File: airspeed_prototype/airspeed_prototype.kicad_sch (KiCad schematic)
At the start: 2 parts, among them U1 BME280, U2 ADXL343

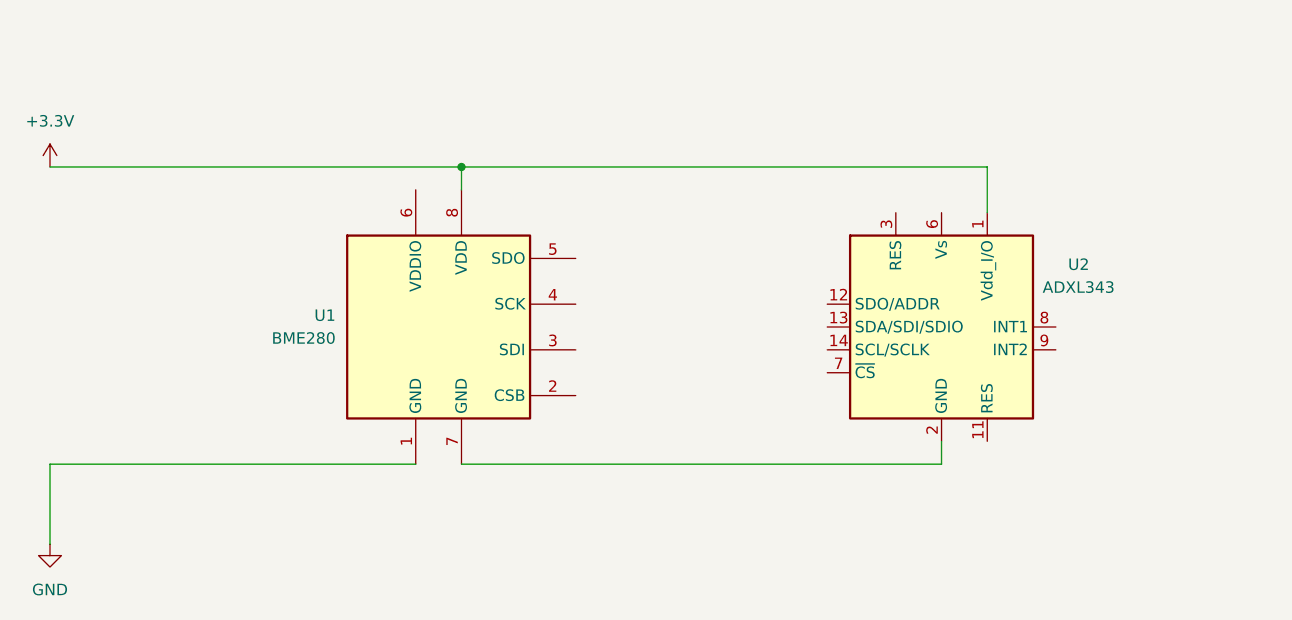
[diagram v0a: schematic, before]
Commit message: schematic
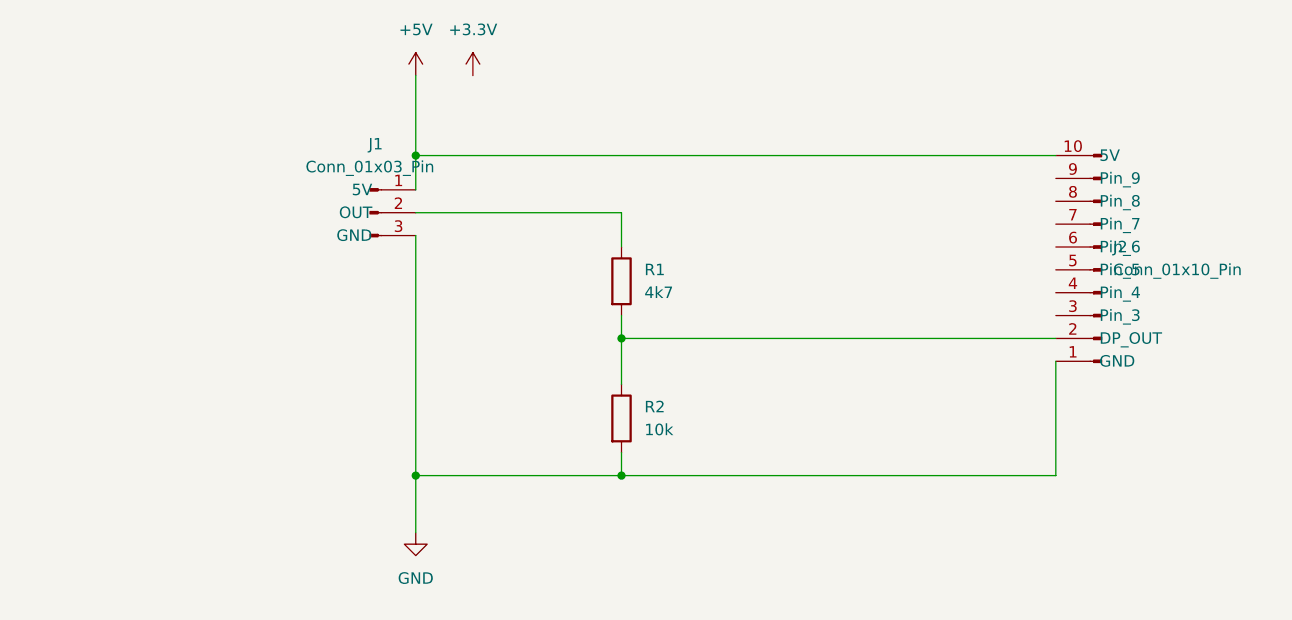
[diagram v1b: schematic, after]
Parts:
- removed U1: BME280, Package_LGA:Bosch_LGA-8_2.5x2.5mm_P0.65mm_ClockwisePinNumbering, symbol Sensor:BME280
- removed U2: ADXL343, Package_LGA:LGA-14_3x5mm_P0.8mm_LayoutBorder1x6y, symbol Sensor_Motion:ADXL343
- added J1: Conn_01x03_Pin, Connector_PinHeader_2.54mm:PinHeader_1x03_P2.54mm_Vertical, symbol Connector:Conn_01x03_Pin
- added J2: Conn_01x10_Pin, Connector_PinHeader_2.54mm:PinHeader_1x10_P2.54mm_Vertical, symbol Connector:Conn_01x10_Pin
- added R1: 4k7, Resistor_SMD:R_0805_2012Metric, symbol Device:R
- added R2: 10k, Resistor_SMD:R_0805_2012Metric, symbol Device:R
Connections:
- net GND: now also J1.3 (Pin_3), J2.1 (Pin_1), R2.2
- new net: J1.2 (Pin_2), R1.1
- new net: J2.2 (Pin_2), R1.2, R2.1
- new net +5V: J1.1 (Pin_1), J2.10 (Pin_10)

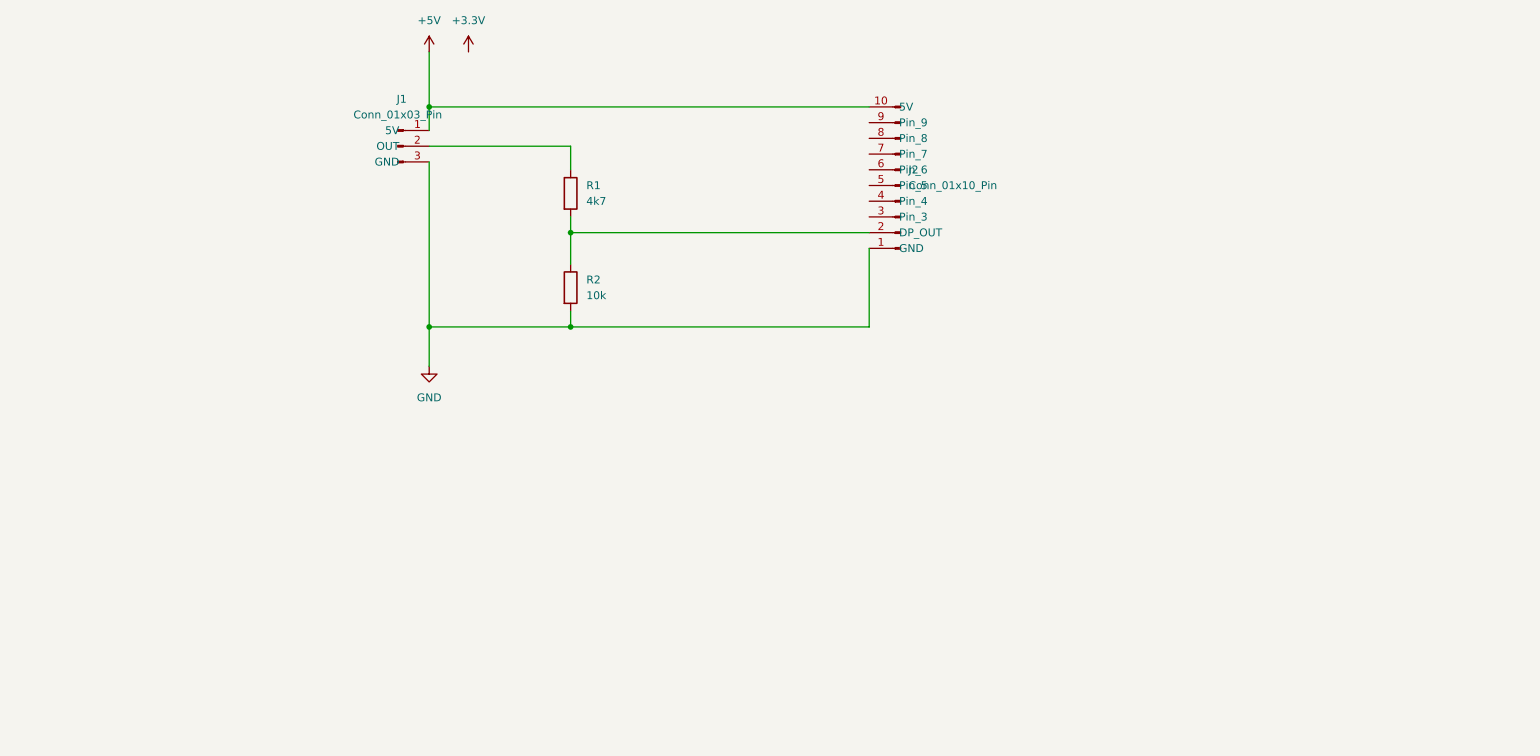
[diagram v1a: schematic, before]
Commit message: update the schematic and pcb
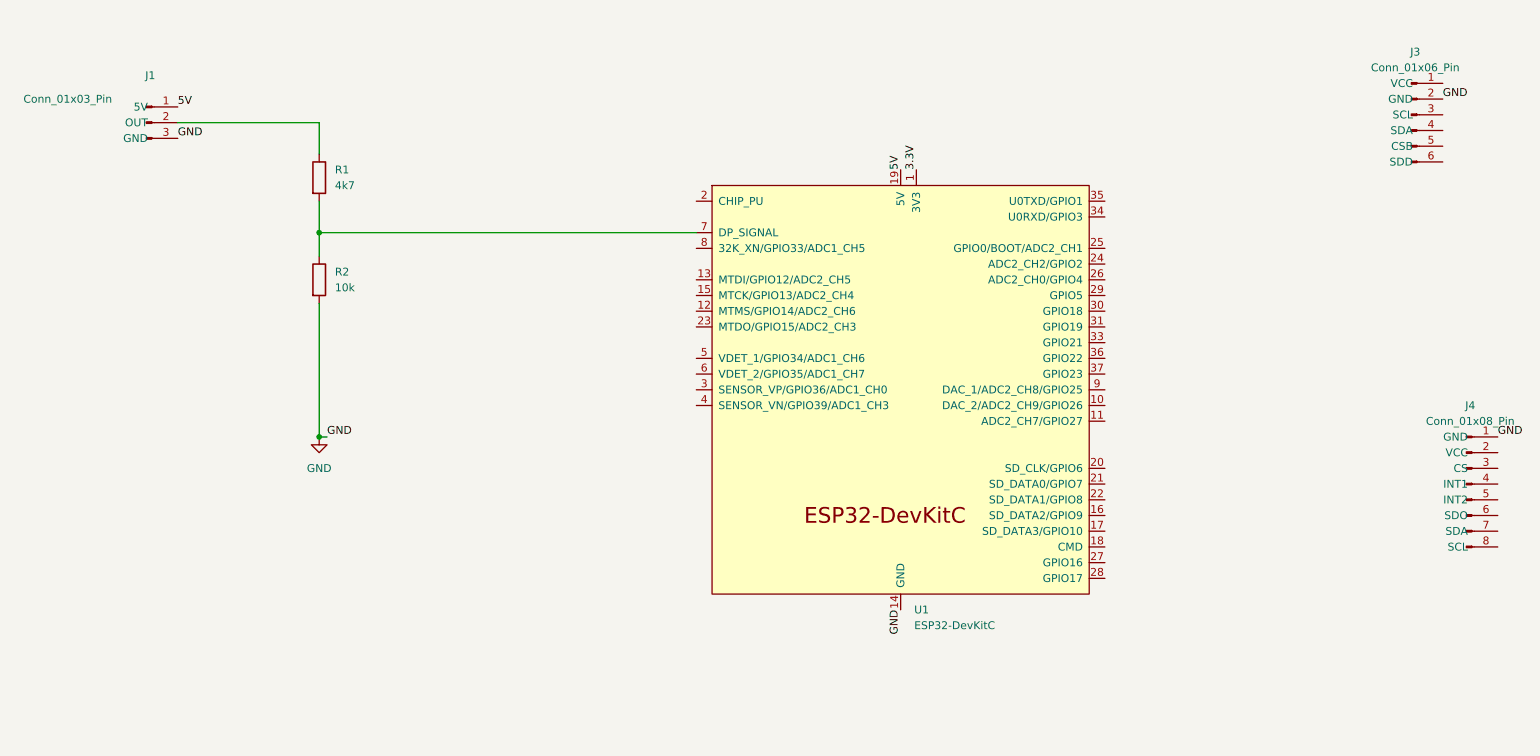
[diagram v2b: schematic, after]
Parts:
- removed J2: Conn_01x10_Pin, Connector_PinHeader_2.54mm:PinHeader_1x10_P2.54mm_Vertical, symbol Connector:Conn_01x10_Pin
- added J3: Conn_01x06_Pin, Connector_PinHeader_2.54mm:PinHeader_1x06_P2.54mm_Vertical, symbol Connector:Conn_01x06_Pin
- added J4: Conn_01x08_Pin, Connector_PinHeader_2.54mm:PinHeader_1x08_P2.54mm_Vertical, symbol Connector:Conn_01x08_Pin
- added U1: ESP32-DevKitC, PCM_Espressif:ESP32-DevKitC, symbol PCM_Espressif:ESP32-DevKitC
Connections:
- net GND: now also J3.2 (GND), J4.1 (GND), U1.14 (GND), U1.32 (GND), U1.38 (GND)
- net at R1.2, R2.1: now also U1.7 (32K_XP/GPIO32/ADC1_CH4)
- net +5V renamed 5V
- net 5V: now also U1.19 (5V)
- new net 3.3V: U1.1 (3V3)
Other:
- moved on the sheet: J1, R1, R2

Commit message: updates
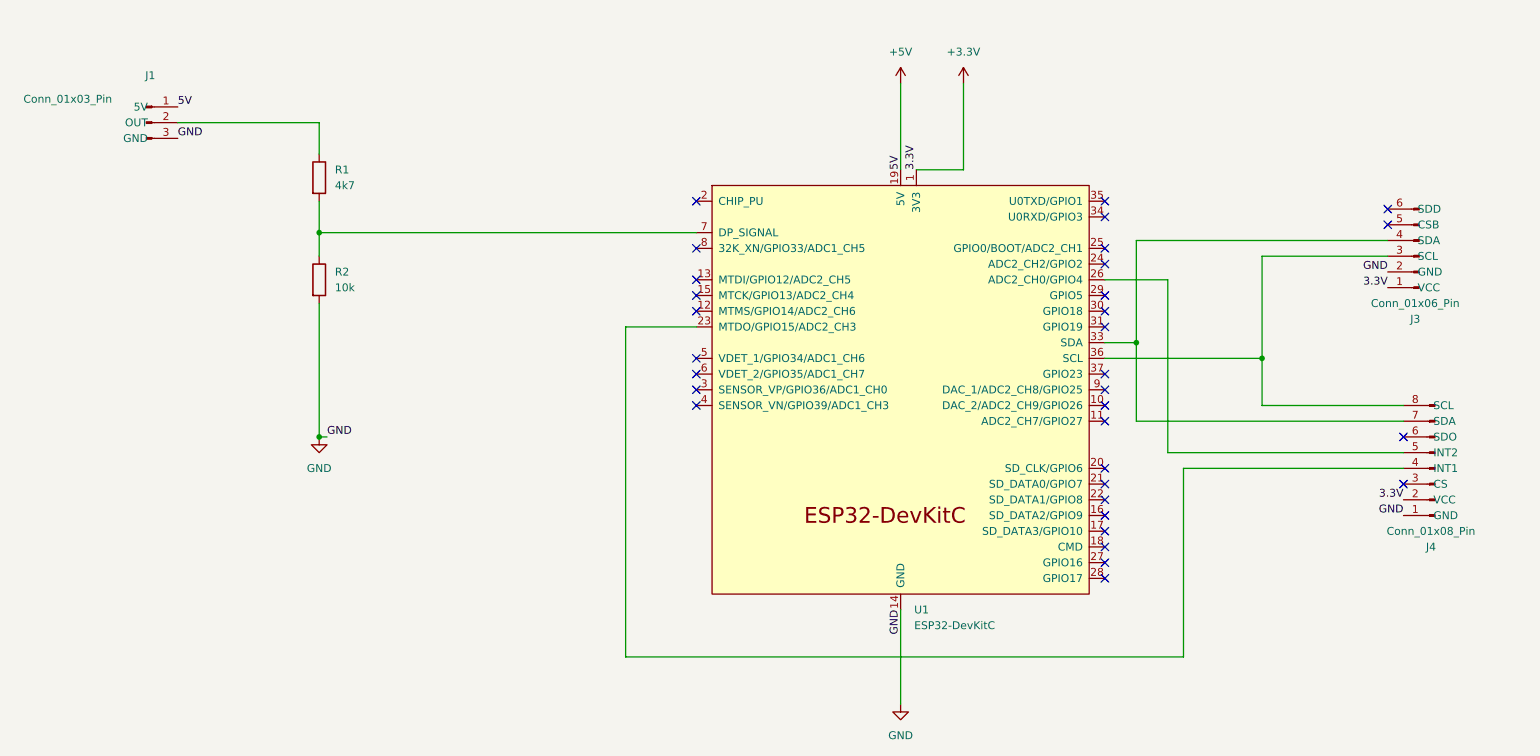
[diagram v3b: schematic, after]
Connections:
- net 3.3V is gone; now on net +3.3V: U1.1 (3V3)
- net at U1.23 (MTDO/GPIO15/ADC2_CH3): now also J4.4 (INT1)
- net at U1.26 (ADC2_CH0/GPIO4): now also J4.5 (INT2)
- net at U1.33 (GPIO21): now also J3.4 (SDA), J4.7 (SDA)
- net at U1.36 (GPIO22): now also J3.3 (SCL), J4.8 (SCL)
- net +3.3V: now reaches J4.2 (VCC)
- net +3.3V: now also J3.1 (VCC)
- net 5V renamed +5V
- no-connect marks 0 -> 32
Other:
- moved on the sheet: J3, J4
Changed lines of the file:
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@@
   (junction (at 68.58 55.88) (diameter 0) (color 0 0 0 0)
   )
+  (junction (at 200.66 73.66) (diameter 0) (color 0 0 0 0)
+  )
+  (junction (at 220.98 76.2) (diameter 0) (color 0 0 0 0)
+  )
   (junction (at 68.58 88.9) (diameter 0) (color 0 0 0 0)
   )
+  (no_connect (at 129.54 68.58))
+  (no_connect (at 129.54 76.2))
+  (no_connect (at 129.54 81.28))
+  (no_connect (at 129.54 50.8))
+  (no_connect (at 195.58 86.36))
+  (no_connect (at 129.54 58.42))
+  (no_connect (at 129.54 63.5))
+  (no_connect (at 195.58 99.06))
+  (no_connect (at 243.84 96.52))
+  (no_connect (at 241.3 54.61))
+  (no_connect (at 241.3 52.07))
+  (no_connect (at 195.58 68.58))
+  (no_connect (at 195.58 53.34))
+  (no_connect (at 195.58 109.22))
+  (no_connect (at 195.58 104.14))
+  (no_connect (at 129.54 83.82))
+  (no_connect (at 195.58 81.28))
+  (no_connect (at 195.58 58.42))
+  (no_connect (at 195.58 83.82))
+  (no_connect (at 195.58 101.6))
+  (no_connect (at 195.58 78.74))
+  (no_connect (at 195.58 93.98))
+  (no_connect (at 129.54 66.04))
+  (no_connect (at 195.58 66.04))
+  (no_connect (at 129.54 78.74))
+  (no_connect (at 195.58 71.12))
+  (no_connect (at 195.58 106.68))
+  (no_connect (at 243.84 88.9))
+  (no_connect (at 195.58 96.52))
+  (no_connect (at 195.58 50.8))
+  (no_connect (at 195.58 60.96))
+  (no_connect (at 195.58 111.76))
+  (wire (pts (xy 162.56 31.75) (xy 162.56 45.72))
+    (stroke (width 0) (type default))
+  )
+  (wire (pts (xy 241.3 59.69) (xy 220.98 59.69))
+    (stroke (width 0) (type default))
+  )
   (wire (pts (xy 68.58 67.31) (xy 68.58 88.9))
     (stroke (width 0) (type default))
   )
+  (wire (pts (xy 208.28 124.46) (xy 118.11 124.46))
+    (stroke (width 0) (type default))
+  )
+  (wire (pts (xy 243.84 83.82) (xy 220.98 83.82))
+    (stroke (width 0) (type default))
+  )
   (wire (pts (xy 129.54 55.88) (xy 68.58 55.88))
     (stroke (width 0) (type default))
   )
+  (wire (pts (xy 162.56 116.84) (xy 162.56 132.08))
+    (stroke (width 0) (type default))
+  )
+  (wire (pts (xy 220.98 76.2) (xy 195.58 76.2))
+    (stroke (width 0) (type default))
+  )
   (wire (pts (xy 69.85 88.9) (xy 68.58 88.9))
     (stroke (width 0) (type default))
   )
+  (wire (pts (xy 243.84 91.44) (xy 205.74 91.44))
+    (stroke (width 0) (type default))
+  )
+  (wire (pts (xy 172.72 31.75) (xy 172.72 45.72))
+    (stroke (width 0) (type default))
+  )
+  (wire (pts (xy 200.66 57.15) (xy 200.66 73.66))
+    (stroke (width 0) (type default))
+  )
+  (wire (pts (xy 205.74 91.44) (xy 205.74 63.5))
+    (stroke (width 0) (type default))
+  )
+  (wire (pts (xy 208.28 93.98) (xy 208.28 124.46))
+    (stroke (width 0) (type default))
+  )
   (wire (pts (xy 45.72 38.1) (xy 68.58 38.1))
     (stroke (width 0) (type default))
   )
+  (wire (pts (xy 200.66 86.36) (xy 243.84 86.36))
+    (stroke (width 0) (type default))
+  )
+  (wire (pts (xy 172.72 45.72) (xy 165.1 45.72))
+    (stroke (width 0) (type default))
+  )
   (wire (pts (xy 68.58 50.8) (xy 68.58 55.88))
     (stroke (width 0) (type default))
   )
+  (wire (pts (xy 241.3 57.15) (xy 200.66 57.15))
+    (stroke (width 0) (type default))
+  )
+  (wire (pts (xy 195.58 63.5) (xy 205.74 63.5))
+    (stroke (width 0) (type default))
+  )
+  (wire (pts (xy 118.11 124.46) (xy 118.11 71.12))
+    (stroke (width 0) (type default))
+  )
+  (wire (pts (xy 243.84 93.98) (xy 208.28 93.98))
+    (stroke (width 0) (type default))
+  )
+  (wire (pts (xy 118.11 71.12) (xy 129.54 71.12))
+    (stroke (width 0) (type default))
+  )
+  (wire (pts (xy 220.98 59.69) (xy 220.98 76.2))
+    (stroke (width 0) (type default))
+  )
   (wire (pts (xy 68.58 55.88) (xy 68.58 59.69))
     (stroke (width 0) (type default))
@@
     (stroke (width 0) (type default))
   )
-  (label "GND" (at 259.08 88.9 0) (fields_autoplaced)
-    (effects (font (size 1.27 1.27)) (justify left bottom))
+  (wire (pts (xy 200.66 73.66) (xy 195.58 73.66))
+    (stroke (width 0) (type default))
+  )
+  (wire (pts (xy 220.98 83.82) (xy 220.98 76.2))
+    (stroke (width 0) (type default))
+  )
+  (wire (pts (xy 200.66 73.66) (xy 200.66 86.36))
+    (stroke (width 0) (type default))
+  )
+  (label "GND" (at 243.84 101.6 180) (fields_autoplaced)
+    (effects (font (size 1.27 1.27)) (justify right bottom))
   )
   (label "3.3V" (at 165.1 45.72 90) (fields_autoplaced)
@@
     (effects (font (size 1.27 1.27)) (justify right bottom))
   )
-  (label "GND" (at 250.19 34.29 0) (fields_autoplaced)
-    (effects (font (size 1.27 1.27)) (justify left bottom))
+  (label "GND" (at 241.3 62.23 180) (fields_autoplaced)
+    (effects (font (size 1.27 1.27)) (justify right bottom))
+  )
+  (label "3.3V" (at 243.84 99.06 180) (fields_autoplaced)
+    (effects (font (size 1.27 1.27)) (justify right bottom))
+  )
+  (label "3.3V" (at 241.3 64.77 180) (fields_autoplaced)
+    (effects (font (size 1.27 1.27)) (justify right bottom))
   )
   (label "GND" (at 69.85 88.9 0) (fields_autoplaced)
@@
     (pin "31")
     (pin "32")
-    (pin "33")
+    (pin "33" (alternate "SDA"))
     (pin "34")
     (pin "35")
-    (pin "36")
+    (pin "36" (alternate "SCL"))
     (pin "37")
     (pin "38")
@@
     )
   )
-  (symbol (lib_id "Connector:Conn_01x08_Pin") (at 254 96.52 0) (unit 1)
-    (in_bom yes) (on_board yes) (dnp no) (fields_autoplaced)
-    (property "Reference" "J4" (at 254.635 83.82 0)
-      (effects (font (size 1.27 1.27)))
-    )
-    (property "Value" "Conn_01x08_Pin" (at 254.635 86.36 0)
-      (effects (font (size 1.27 1.27)))
-    )
-    (property "Footprint" "Connector_PinHeader_2.54mm:PinHeader_1x08_P2.54mm_Vertical" (at 254 96.52 0)
-      (effects (font (size 1.27 1.27)) hide)
-    )
-    (property "Datasheet" "~" (at 254 96.52 0)
+  (symbol (lib_id "Connector:Conn_01x08_Pin") (at 248.92 93.98 180) (unit 1)
+    (in_bom yes) (on_board yes) (dnp no) (fields_autoplaced)
+    (property "Reference" "J4" (at 248.285 106.68 0)
+      (effects (font (size 1.27 1.27)))
+    )
+    (property "Value" "Conn_01x08_Pin" (at 248.285 104.14 0)
+      (effects (font (size 1.27 1.27)))
+    )
+    (property "Footprint" "Connector_PinHeader_2.54mm:PinHeader_1x08_P2.54mm_Vertical" (at 248.92 93.98 0)
+      (effects (font (size 1.27 1.27)) hide)
+    )
+    (property "Datasheet" "~" (at 248.92 93.98 0)
       (effects (font (size 1.27 1.27)) hide)
     )
@@
     )
   )
-  (symbol (lib_id "Connector:Conn_01x06_Pin") (at 245.11 36.83 0) (unit 1)
-    (in_bom yes) (on_board yes) (dnp no) (fields_autoplaced)
-    (property "Reference" "J3" (at 245.745 26.67 0)
-      (effects (font (size 1.27 1.27)))
-    )
-    (property "Value" "Conn_01x06_Pin" (at 245.745 29.21 0)
-      (effects (font (size 1.27 1.27)))
-    )
-    (property "Footprint" "Connector_PinHeader_2.54mm:PinHeader_1x06_P2.54mm_Vertical" (at 245.11 36.83 0)
-      (effects (font (size 1.27 1.27)) hide)
-    )
-    (property "Datasheet" "~" (at 245.11 36.83 0)
+  (symbol (lib_id "power:+3.3V") (at 172.72 31.75 0) (unit 1)
+    (in_bom yes) (on_board yes) (dnp no)
+    (property "Reference" "#PWR04" (at 172.72 35.56 0)
+      (effects (font (size 1.27 1.27)) hide)
+    )
+    (property "Value" "+3.3V" (at 172.72 26.67 0)
+      (effects (font (size 1.27 1.27)))
+    )
+    (property "Footprint" "" (at 172.72 31.75 0)
+      (effects (font (size 1.27 1.27)) hide)
+    )
+    (property "Datasheet" "" (at 172.72 31.75 0)
+      (effects (font (size 1.27 1.27)) hide)
+    )
+    (pin "1")
+    (instances
+      (project "airspeed_prototype"
+        (path "/2dd51ea1-493d-49cb-b057-63d48ce841c4"
+          (reference "#PWR04") (unit 1)
+        )
+      )
+    )
+  )
+  (symbol (lib_id "Connector:Conn_01x06_Pin") (at 246.38 59.69 180) (unit 1)
+    (in_bom yes) (on_board yes) (dnp no) (fields_autoplaced)
+    (property "Reference" "J3" (at 245.745 69.85 0)
+      (effects (font (size 1.27 1.27)))
+    )
+    (property "Value" "Conn_01x06_Pin" (at 245.745 67.31 0)
+      (effects (font (size 1.27 1.27)))
+    )
+    (property "Footprint" "Connector_PinHeader_2.54mm:PinHeader_1x06_P2.54mm_Vertical" (at 246.38 59.69 0)
+      (effects (font (size 1.27 1.27)) hide)
+    )
+    (property "Datasheet" "~" (at 246.38 59.69 0)
       (effects (font (size 1.27 1.27)) hide)
     )
@@
     )
   )
+  (symbol (lib_id "power:+5V") (at 162.56 31.75 0) (unit 1)
+    (in_bom yes) (on_board yes) (dnp no) (fields_autoplaced)
+    (property "Reference" "#PWR03" (at 162.56 35.56 0)
+      (effects (font (size 1.27 1.27)) hide)
+    )
+    (property "Value" "+5V" (at 162.56 26.67 0)
+      (effects (font (size 1.27 1.27)))
+    )
+    (property "Footprint" "" (at 162.56 31.75 0)
+      (effects (font (size 1.27 1.27)) hide)
+    )
+    (property "Datasheet" "" (at 162.56 31.75 0)
+      (effects (font (size 1.27 1.27)) hide)
+    )
+    (pin "1")
+    (instances
+      (project "airspeed_prototype"
+        (path "/2dd51ea1-493d-49cb-b057-63d48ce841c4"
+          (reference "#PWR03") (unit 1)
+        )
+      )
+    )
+  )
   (symbol (lib_id "Device:R") (at 68.58 46.99 0) (unit 1)
     (in_bom yes) (on_board yes) (dnp no) (fields_autoplaced)
@@
         )
       )
+    )
+  )
+  (symbol (lib_id "power:GND") (at 162.56 132.08 0) (unit 1)
+    (in_bom yes) (on_board yes) (dnp no) (fields_autoplaced)
+    (property "Reference" "#PWR02" (at 162.56 138.43 0)
+      (effects (font (size 1.27 1.27)) hide)
+    )
+    (property "Value" "GND" (at 162.56 137.16 0)
+      (effects (font (size 1.27 1.27)))
+    )
+    (property "Footprint" "" (at 162.56 132.08 0)
+      (effects (font (size 1.27 1.27)) hide)
+    )
+    (property "Datasheet" "" (at 162.56 132.08 0)
+      (effects (font (size 1.27 1.27)) hide)
+    )
+    (pin "1")
+    (instances
+      (project "airspeed_prototype"
+        (path "/2dd51ea1-493d-49cb-b057-63d48ce841c4"
+          (reference "#PWR02") (unit 1)
+        )
+      )
